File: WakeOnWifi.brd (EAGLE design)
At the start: 85 x 45 mm, 15 parts

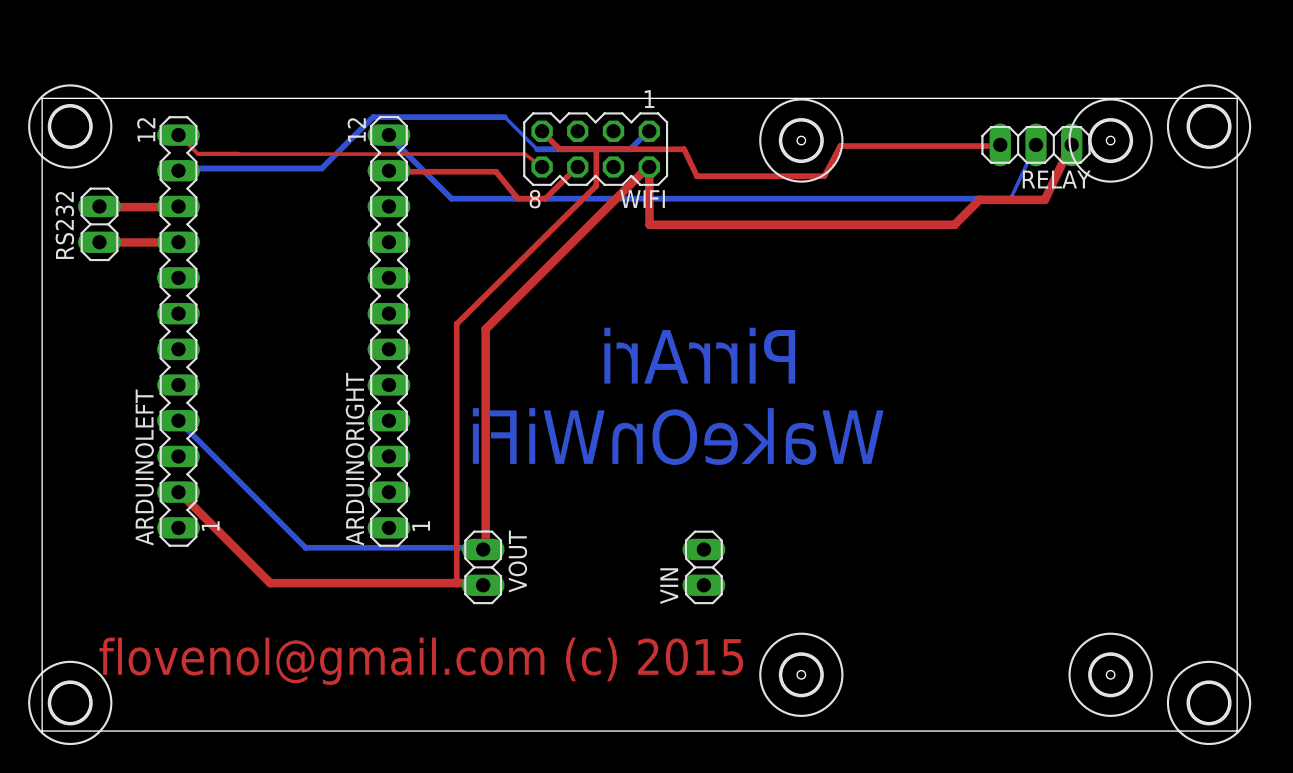
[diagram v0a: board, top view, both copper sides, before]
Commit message: WakeOnWifi board fixes
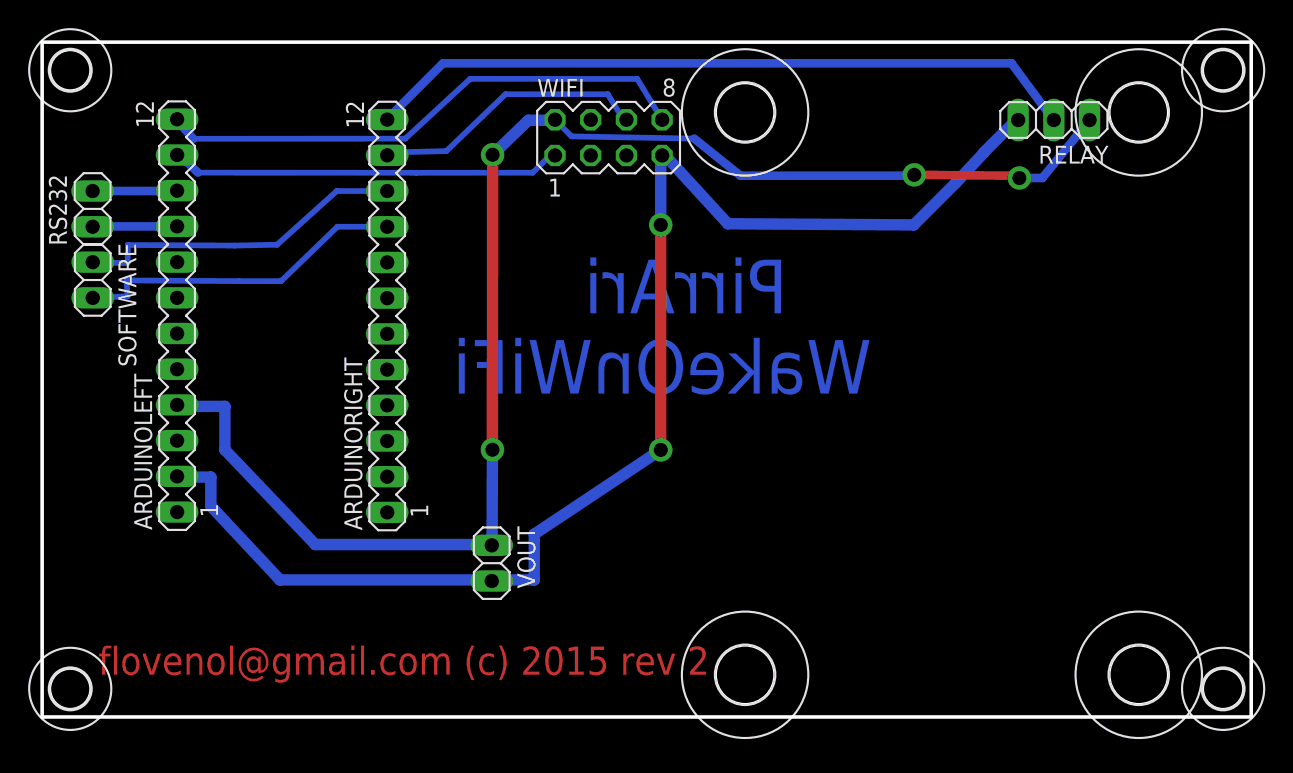
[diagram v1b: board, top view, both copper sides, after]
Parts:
- removed VIN: (no value), pinhead:1X02
- added SOFTWARE: (no value), pinhead:1X02
- U$5, U$6, U$7, U$8: device holes:2,8 -> holes:4,1
- moved U$1 85.6 mm to (2.00, 79.0)
- moved U$5 76.0 mm to (78.0, 76.0)
- moved U$4 65.0 mm to (2.00, 35.0)
- moved U$6 63.8 mm to (50.0, 76.0)
- moved U$2 52.4 mm to (84.0, 79.0)
- moved U$8 51.1 mm to (50.0, 36.0)
- moved U$3 39.8 mm to (84.0, 35.0)
- moved U$7 5.39 mm to (78.0, 36.0)
- moved RELAY 2.18 mm to (72.0, 75.5)
- moved WIFI 1.23 mm to (40.3, 74.2), turned to 0 degrees
- moved RS232 1.20 mm to (3.59, 69.1)
- moved ARDUINOLEFT 1.13 mm to (9.60, 61.5)
- moved ARDUINORIGHT 1.11 mm to (24.5, 61.5)
- moved VOUT 0.68 mm to (32.0, 43.9)
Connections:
- removed net +5V: VIN.1
- removed net GND: VIN.2
- new net N$6: ARDUINORIGHT.10, SOFTWARE.1
- new net N$7: ARDUINORIGHT.9, SOFTWARE.2
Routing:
- net N$7: track 0.00 -> 23.7 mm
- net N$6: track 0.00 -> 23.7 mm
- net N$2: track 28.7 -> 38.6 mm
- net N$4: track 95.1 -> 103.5 mm, vias 0 -> 4
- net N$3: track 36.5 -> 28.3 mm
- net N$5: track 15.3 -> 19.8 mm
- net N$1: track 95.3 -> 96.2 mm, vias 0 -> 2
- net N$8: track 50.4 -> 51.1 mm
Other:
- board size 85 x 45 mm -> 86 x 48 mm
- board text added: "flovenol@gmail.com (c) 2015 rev 2"
- board text removed: "flovenol@gmail.com (c) 2015"
